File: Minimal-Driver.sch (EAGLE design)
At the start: 8 parts, among them J3 6p-2.54, M1 MOTOR_PADS, Q1 CJ2302

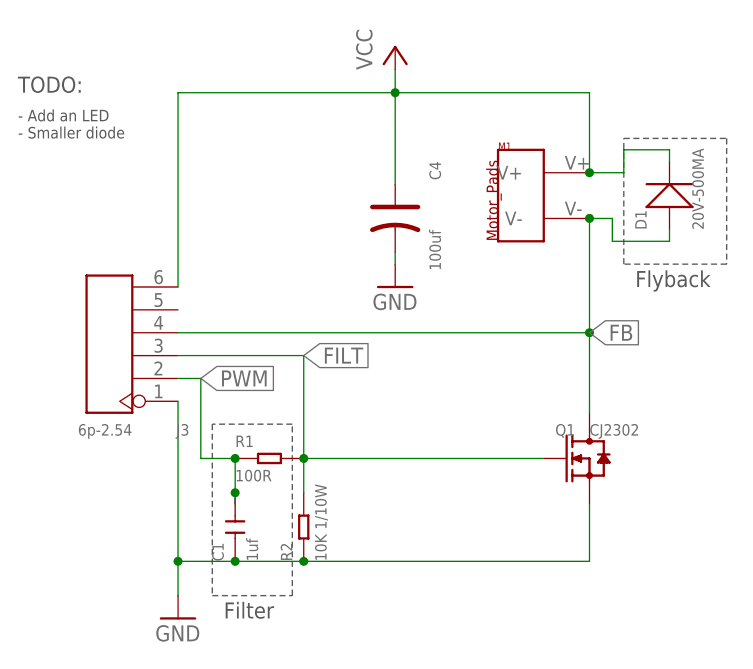
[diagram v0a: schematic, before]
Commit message: cleanup
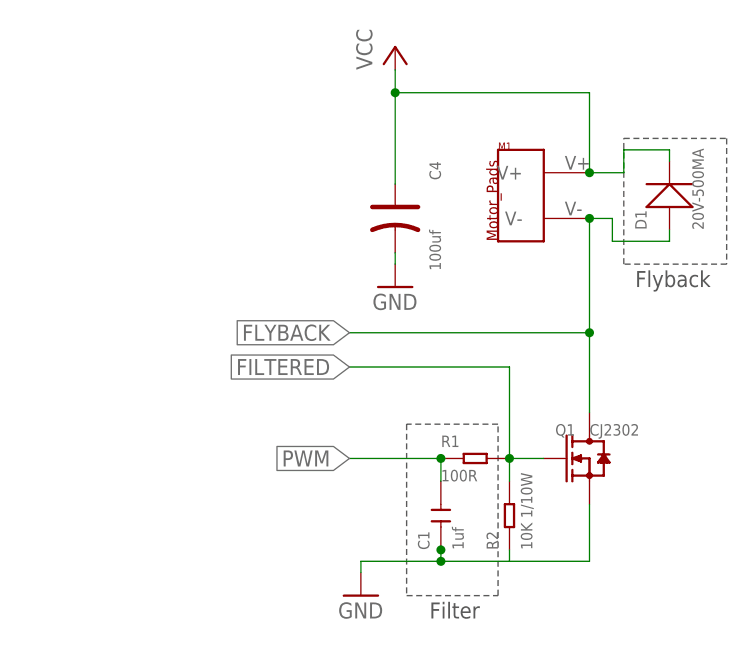
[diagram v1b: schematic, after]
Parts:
- removed J3: 6p-2.54, Seeed-Connector -2016:DIP-BLACK-MALE-HEADER(6P-2.54)
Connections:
- removed net FB: D1.+, J3.4, M1.V-, Q1.D
- removed net FILT: J3.3, Q1.G, R1.2, R2.2
- new net FILTERED: Q1.G, R1.2, R2.2
- new net FLYBACK: D1.+, M1.V-, Q1.D
- net GND: no longer J3.1
- net PWM: no longer J3.2
- net VCC: no longer J3.6
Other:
- note removed: "- Add an LED - Smaller diode"
- note removed: "TODO:"
- moved on the sheet: C1, R1, R2
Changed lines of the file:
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@@
 <part name="D1" library="Seeed-Diode-2016" deviceset="SMD-DIODE-SCHOTTKY-20V-500MA(SOD-123)" device="" value="20V-500MA"/>
 <part name="FRAME1" library="frames" deviceset="FRAME_A_L" device=""/>
-<part name="J3" library="Seeed-Connector -2016" deviceset="DIP-BLACK-MALE-HEADER(6P-2.54)" device="" value="6p-2.54"/>
 </parts>
 <sheets>
 <sheet>
 <plain>
-<text x="83.82" y="139.7" size="1.778" layer="97">TODO:</text>
-<text x="83.82" y="134.62" size="1.27" layer="97">- Add an LED
-- Smaller diode</text>
-<wire x1="105.41" y1="102.87" x2="105.41" y2="83.82" width="0.1524" layer="97" style="shortdash"/>
-<wire x1="105.41" y1="83.82" x2="114.3" y2="83.82" width="0.1524" layer="97" style="shortdash"/>
-<wire x1="114.3" y1="83.82" x2="114.3" y2="102.87" width="0.1524" layer="97" style="shortdash"/>
-<wire x1="114.3" y1="102.87" x2="105.41" y2="102.87" width="0.1524" layer="97" style="shortdash"/>
-<text x="106.68" y="81.28" size="1.778" layer="97">Filter</text>
+<wire x1="127" y1="102.87" x2="127" y2="83.82" width="0.1524" layer="97" style="shortdash"/>
+<wire x1="127" y1="83.82" x2="137.16" y2="83.82" width="0.1524" layer="97" style="shortdash"/>
+<wire x1="137.16" y1="83.82" x2="137.16" y2="102.87" width="0.1524" layer="97" style="shortdash"/>
+<wire x1="137.16" y1="102.87" x2="127" y2="102.87" width="0.1524" layer="97" style="shortdash"/>
+<text x="129.54" y="81.28" size="1.778" layer="97">Filter</text>
 <wire x1="151.13" y1="134.62" x2="162.56" y2="134.62" width="0.1524" layer="97" style="shortdash"/>
 <wire x1="162.56" y1="134.62" x2="162.56" y2="120.65" width="0.1524" layer="97" style="shortdash"/>
@@
 <instances>
 <instance part="Q1" gate="G$1" x="147.32" y="99.06"/>
-<instance part="R1" gate="G$1" x="111.76" y="99.06"/>
-<instance part="R2" gate="G$1" x="115.57" y="91.44" rot="R90"/>
-<instance part="C1" gate="G$1" x="107.95" y="91.44" rot="R90"/>
+<instance part="R1" gate="G$1" x="134.62" y="99.06"/>
+<instance part="R2" gate="G$1" x="138.43" y="92.71" rot="R90"/>
+<instance part="C1" gate="G$1" x="130.81" y="92.71" rot="R90"/>
 <instance part="C4" gate="G$1" x="125.73" y="125.73" rot="R270"/>
-<instance part="GND1" gate="1" x="101.6" y="81.28"/>
+<instance part="GND1" gate="1" x="121.92" y="83.82"/>
 <instance part="GND2" gate="1" x="125.73" y="118.11"/>
 <instance part="P+1" gate="VCC" x="125.73" y="144.78"/>
@@
 <instance part="FRAME1" gate="G$1" x="0" y="0"/>
 <instance part="FRAME1" gate="G$2" x="172.72" y="0"/>
-<instance part="J3" gate="G$1" x="93.98" y="111.76" rot="R180"/>
 </instances>
 <busses>
@@
 <pinref part="R2" gate="G$1" pin="1"/>
 <pinref part="C1" gate="G$1" pin="1"/>
-<wire x1="147.32" y1="87.63" x2="115.57" y2="87.63" width="0.1524" layer="91"/>
-<wire x1="115.57" y1="87.63" x2="107.95" y2="87.63" width="0.1524" layer="91"/>
-<junction x="115.57" y="87.63"/>
+<junction x="130.81" y="88.9"/>
+<wire x1="130.81" y1="87.63" x2="130.81" y2="88.9" width="0.1524" layer="91"/>
+<junction x="130.81" y="87.63"/>
 <pinref part="GND1" gate="1" pin="GND"/>
-<wire x1="107.95" y1="87.63" x2="101.6" y2="87.63" width="0.1524" layer="91"/>
-<wire x1="101.6" y1="87.63" x2="101.6" y2="83.82" width="0.1524" layer="91"/>
-<junction x="107.95" y="87.63"/>
-<junction x="101.6" y="87.63"/>
-<wire x1="101.6" y1="87.63" x2="101.6" y2="105.41" width="0.1524" layer="91"/>
-<pinref part="J3" gate="G$1" pin="1"/>
+<wire x1="121.92" y1="86.36" x2="121.92" y2="87.63" width="0.1524" layer="91"/>
+<wire x1="121.92" y1="87.63" x2="130.81" y2="87.63" width="0.1524" layer="91"/>
+<wire x1="130.81" y1="87.63" x2="138.43" y2="87.63" width="0.1524" layer="91"/>
+<wire x1="138.43" y1="88.9" x2="138.43" y2="87.63" width="0.1524" layer="91"/>
+<wire x1="138.43" y1="87.63" x2="147.32" y2="87.63" width="0.1524" layer="91"/>
 </segment>
 </net>
@@
 <junction x="147.32" y="130.81"/>
 <wire x1="151.13" y1="133.35" x2="156.21" y2="133.35" width="0.1524" layer="91"/>
-<wire x1="125.73" y1="139.7" x2="101.6" y2="139.7" width="0.1524" layer="91"/>
-<wire x1="101.6" y1="139.7" x2="101.6" y2="118.11" width="0.1524" layer="91"/>
-<pinref part="J3" gate="G$1" pin="6"/>
 <pinref part="C4" gate="G$1" pin="+"/>
 <wire x1="125.73" y1="139.7" x2="125.73" y2="129.54" width="0.1524" layer="91"/>
@@
 <segment>
 <pinref part="R1" gate="G$1" pin="1"/>
-<wire x1="107.95" y1="93.98" x2="107.95" y2="95.25" width="0.1524" layer="91"/>
-<wire x1="107.95" y1="95.25" x2="107.95" y2="99.06" width="0.1524" layer="91"/>
-<junction x="107.95" y="99.06"/>
+<wire x1="130.81" y1="96.52" x2="130.81" y2="99.06" width="0.1524" layer="91"/>
+<junction x="130.81" y="99.06"/>
 <pinref part="C1" gate="G$1" pin="2"/>
-<junction x="107.95" y="95.25"/>
-<wire x1="104.14" y1="99.06" x2="107.95" y2="99.06" width="0.1524" layer="91"/>
-<wire x1="101.6" y1="107.95" x2="104.14" y2="107.95" width="0.1524" layer="91"/>
-<wire x1="104.14" y1="107.95" x2="104.14" y2="99.06" width="0.1524" layer="91"/>
-<pinref part="J3" gate="G$1" pin="2"/>
-<label x="104.14" y="107.95" size="1.778" layer="95" xref="yes"/>
+<wire x1="120.65" y1="99.06" x2="130.81" y2="99.06" width="0.1524" layer="91"/>
+<label x="120.65" y="99.06" size="1.778" layer="95" rot="R180" xref="yes"/>
 </segment>
 </net>
-<net name="FILT" class="0">
+<net name="FILTERED" class="0">
 <segment>
 <pinref part="R1" gate="G$1" pin="2"/>
 <pinref part="R2" gate="G$1" pin="2"/>
-<wire x1="115.57" y1="99.06" x2="115.57" y2="95.25" width="0.1524" layer="91"/>
+<wire x1="138.43" y1="99.06" x2="138.43" y2="96.52" width="0.1524" layer="91"/>
 <pinref part="Q1" gate="G$1" pin="G"/>
-<junction x="115.57" y="99.06"/>
-<pinref part="J3" gate="G$1" pin="3"/>
-<wire x1="115.57" y1="99.06" x2="142.24" y2="99.06" width="0.1524" layer="91"/>
-<wire x1="115.57" y1="99.06" x2="115.57" y2="110.49" width="0.1524" layer="91"/>
-<wire x1="115.57" y1="110.49" x2="101.6" y2="110.49" width="0.1524" layer="91"/>
-<label x="115.57" y="110.49" size="1.778" layer="95" xref="yes"/>
+<junction x="138.43" y="99.06"/>
+<wire x1="138.43" y1="99.06" x2="142.24" y2="99.06" width="0.1524" layer="91"/>
+<wire x1="138.43" y1="99.06" x2="138.43" y2="109.22" width="0.1524" layer="91"/>
+<wire x1="138.43" y1="109.22" x2="120.65" y2="109.22" width="0.1524" layer="91"/>
+<label x="120.65" y="109.22" size="1.778" layer="95" rot="R180" xref="yes"/>
 </segment>
 </net>
-<net name="FB" class="1">
+<net name="FLYBACK" class="1">
 <segment>
 <pinref part="D1" gate="G$1" pin="+"/>
@@
 <wire x1="149.86" y1="125.73" x2="147.32" y2="125.73" width="0.1524" layer="91"/>
 <junction x="147.32" y="125.73"/>
-<pinref part="J3" gate="G$1" pin="4"/>
-<wire x1="101.6" y1="113.03" x2="147.32" y2="113.03" width="0.1524" layer="91"/>
+<wire x1="120.65" y1="113.03" x2="147.32" y2="113.03" width="0.1524" layer="91"/>
 <junction x="147.32" y="113.03"/>
-<label x="147.32" y="113.03" size="1.778" layer="95" xref="yes"/>
+<label x="120.65" y="113.03" size="1.778" layer="95" rot="R180" xref="yes"/>
 </segment>
 </net>
@@
 </schematic>
 </drawing>
-<compatibility>
-<note version="6.3" minversion="6.2.2" severity="warning">
-Since Version 6.2.2 text objects can contain more than one line,
-which will not be processed correctly with this version.
-</note>
-</compatibility>
 </eagle>
